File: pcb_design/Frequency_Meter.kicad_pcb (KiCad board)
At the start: 4 copper layers, 52.8 x 38.2 mm, 67 parts, among them IC2 AD8611ARZ, IC3 74LVC1G74DC,125, IC4 AD8021ARZ, IC6 STM32G431KBT6, IC7 REF3125AIDBZT, J2 USB4105-GF-A, J3 Conn_01x04_Pin, J4 RF2-03E-T-00-50-G, U1 USBLC6-2SC6, U2 AP2112K-3.3, Y1 ABM3B-16.000MHZ-10-1-U-T

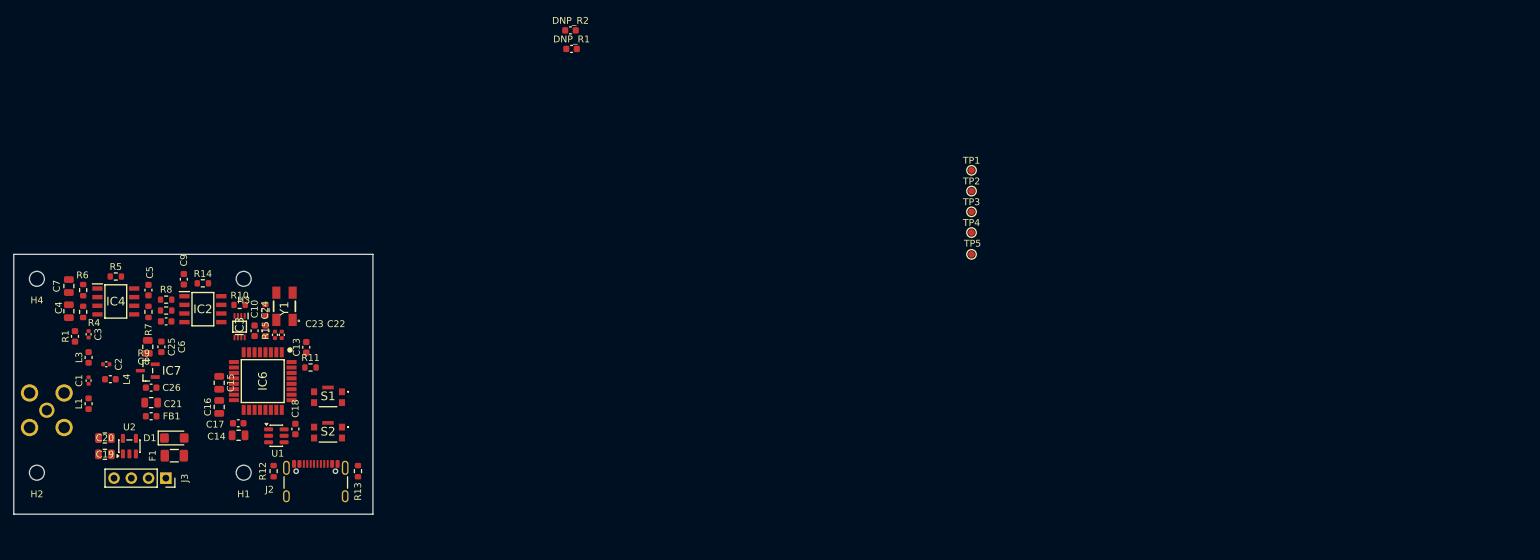
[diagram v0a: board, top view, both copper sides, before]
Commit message: PCB update
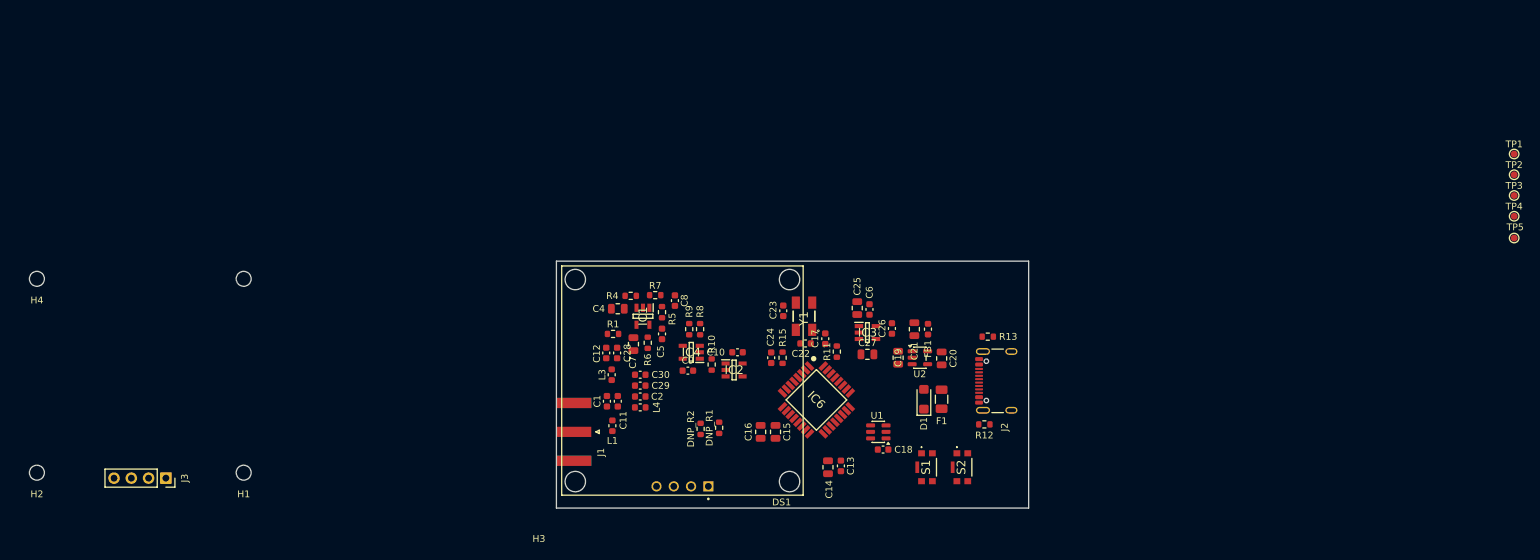
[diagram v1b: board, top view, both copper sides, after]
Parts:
- removed C3: 33pF, Capacitor_SMD:C_0402_1005Metric
- removed IC7: REF3125AIDBZT, FreqMeter:SOT95P237X112-3N
- removed J4: RF2-03E-T-00-50-G, FreqMeter:RF203ET0050G
- removed R14: 330k, Resistor_SMD:R_0603_1608Metric
- added C11: 18pF, Capacitor_SMD:C_0603_1608Metric, F.Cu at (117.8, 115.6)
- added C12: 15pF, Capacitor_SMD:C_0603_1608Metric, F.Cu at (116.1, 108.5)
- added C27: 1uF X7R, Capacitor_SMD:C_0805_2012Metric, F.Cu at (154.5, 108.7)
- added C28: 18pF, Capacitor_SMD:C_0603_1608Metric, F.Cu at (117.7, 108.5)
- added C29: 15pF, Capacitor_SMD:C_0603_1608Metric, F.Cu at (121.1, 113.3)
- added C30: 15pF, Capacitor_SMD:C_0603_1608Metric, F.Cu at (121.1, 111.7)
- added DS1: OLED_128X64_1.3_I2C, Screens:LCD_OLED_128X64_1.3_I2C, F.Cu at (127.3, 112.6)
- added IC1: LMH6629MF_NOPB, FreqMeter:SOT95P280X145-5N, F.Cu at (121.5, 103.1)
- added J1: SMA female 50Ω edge mount, Connector_Coaxial:SMA_Amphenol_132289_EdgeMount, F.Cu at (111.4, 120.1)
- C1: value 33pF -> 15pF; footprint Capacitor_SMD:C_0402_1005Metric -> Capacitor_SMD:C_0603_1608Metric
- C2: value 130pF -> 100pF; footprint Capacitor_SMD:C_0402_1005Metric -> Capacitor_SMD:C_0603_1608Metric
- C22, C23: footprint Capacitor_SMD:C_0402_1005Metric -> Capacitor_SMD:C_0603_1608Metric
- DNP_R1, DNP_R2, R1: footprint Capacitor_SMD:C_0603_1608Metric -> Resistor_SMD:R_0603_1608Metric
- IC2: value AD8611ARZ -> SN74LVC1G80DBVR; footprint FreqMeter:SOIC127P600X175-8N -> FreqMeter:SOT95P280X145-5N
- IC3: value 74LVC1G74DC,125 -> REF2033AIDDCT; footprint FreqMeter:SOP50P310X100-8N -> FreqMeter:SOT95P280X110-5N
- IC4: value AD8021ARZ -> TLV3601DBVR; footprint BSG7:SOIC127P600X175-8N -> FreqMeter:SOT95P280X145-5N
- R10: value 33 Ohm -> 33
- R4: value 10k -> 1k
- R5: value 249 -> 374
- moved C20 123.6 mm to (165.4, 109.3), turned to 90 degrees
- moved C19 117.5 mm to (159.0, 109.2), turned to 90 degrees
- moved U2 116.9 mm to (162.2, 109.2), turned to 0 degrees
- moved FB1 114.9 mm to (163.4, 105.0), turned to 90 degrees
- moved F1 113.1 mm to (165.4, 115.3), turned to 90 degrees
- moved C21 112.7 mm to (161.4, 105.0), turned to -90 degrees
- moved D1 110.3 mm to (162.8, 115.3), turned to 90 degrees
- moved C26 109.2 mm to (158.1, 104.9), turned to 90 degrees
- moved R12 104.7 mm to (171.7, 119.0), turned to 0 degrees
- moved C25 104.5 mm to (153.0, 101.9)
- moved C6 104.2 mm to (154.8, 102.1)
- moved J2 102.4 mm to (174.6, 112.6), turned to 90 degrees
- moved R13 94.7 mm to (172.2, 106.1), turned to 180 degrees
- moved S2 93.4 mm to (168.4, 125.3), turned to 90 degrees
- moved IC3 92.3 mm to (154.5, 105.5), turned to 0 degrees
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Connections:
- C21 pad 1: /RF_5V -> /RF_3V3
- C25 pad 1: /VREF_2V5 -> /VREF_1V6
- C26 pad 1: /RF_5V -> /POWER_5V
- C4 pad 2: /+IN -> /AMP_+IN
- C5 pad 2: /RF_5V -> /RF_3V3
- C6 pad 1: /VREF_2V5 -> /VREF_1V6
- C8 pad 1: /-_NODE -> /COMPARATOR_IN-
- C9 pad 1: GND -> /POWER_3V3
- C9 pad 2: /RF_5V -> GND
- FB1 pad 1: /POWER_5V -> /POWER_3V3
- FB1 pad 2: /RF_5V -> /RF_3V3
- IC2 pad 1: /RF_5V -> /CLK_DIV2
- IC2 pad 2: /COMPARATOR_IN+ -> /CLK_100M
- IC2 pad 3: /-_NODE -> GND
- IC2 pad 4: GND -> /CLK_DIV2
- IC2 pad 5: GND -> /POWER_3V3
- IC3 pad 1: /CLK_100M -> /VREF_1V6
- IC3 pad 2: Net-(IC3-D) -> GND
- IC3 pad 3: Net-(IC3-D) -> /POWER_5V
- IC3 pad 4: GND -> /POWER_5V
- IC3 pad 5: /CLK_DIV2 -> unconnected-(IC3-VREF-Pad5)
- IC4 pad 1: GND -> Net-(IC4-OUT)
- IC4 pad 2: /LOOPBACK- -> GND
- IC4 pad 3: /+IN -> Net-(IC4-IN+)
- IC4 pad 4: GND -> /COMPARATOR_IN-
- IC4 pad 5: unconnected-(IC4-CCOMP-Pad5) -> /POWER_3V3
- R10 pad 1: Net-(IC2-QA) -> Net-(IC4-OUT)
- R4 pad 1: /VREF_2V5 -> /VREF_1V6
- R4 pad 2: /+IN -> /AMP_+IN
- R5 pad 1: /LOOPBACK- -> /AMP_-IN
- R5 pad 2: /LOOPBACK+ -> /AMP_OUT
- R6 pad 1: /LOOPBACK- -> /AMP_-IN
- R7 pad 1: /LOOPBACK+ -> /AMP_OUT
- R8 pad 1: /VREF_2V5 -> /VREF_1V6
- R8 pad 2: /COMPARATOR_IN+ -> Net-(IC4-IN+)
- R9 pad 1: /VREF_2V5 -> /VREF_1V6
- R9 pad 2: /-_NODE -> /COMPARATOR_IN-
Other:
- board size 52.8 x 38.2 mm -> 69.4 x 36.3 mm
